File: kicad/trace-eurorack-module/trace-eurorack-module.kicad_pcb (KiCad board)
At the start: 2 copper layers, 7 parts, among them J1 Eurorack_Power, U1 AP63203WU-7

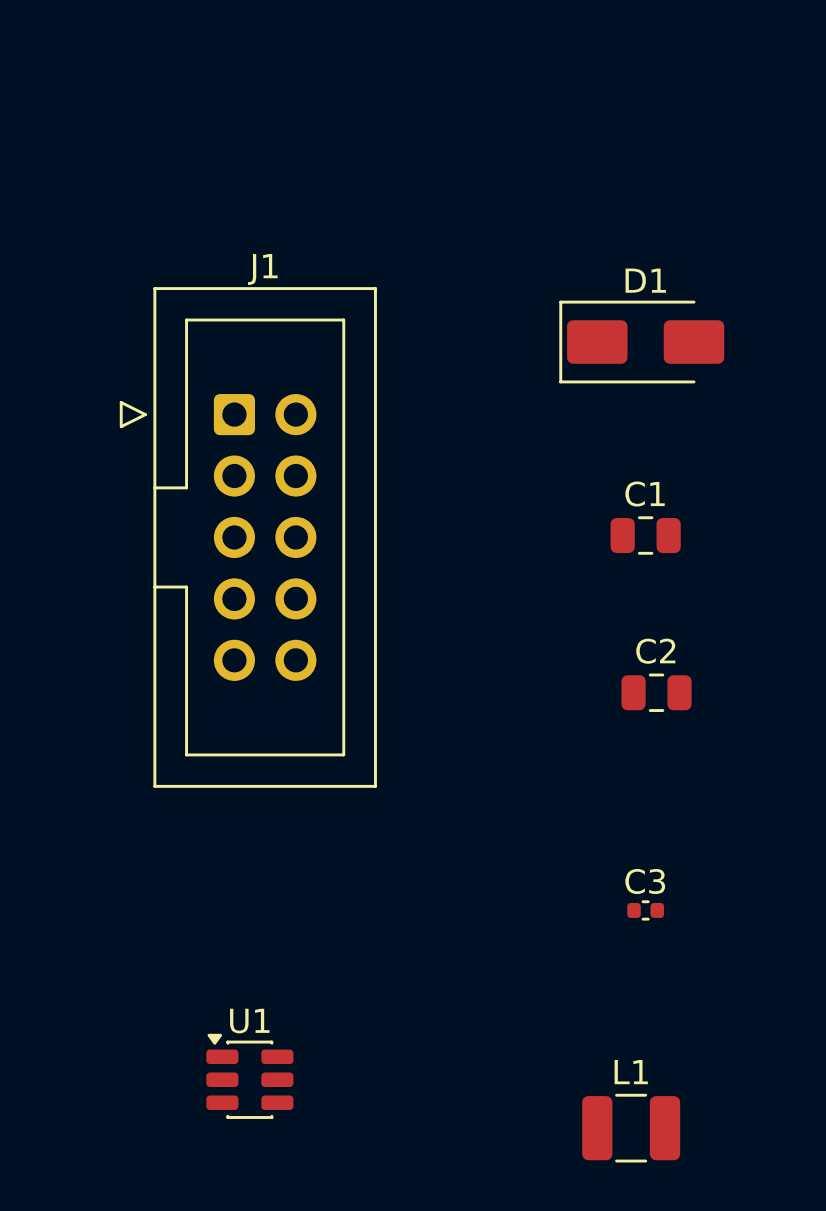
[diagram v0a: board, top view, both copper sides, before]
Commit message: saved
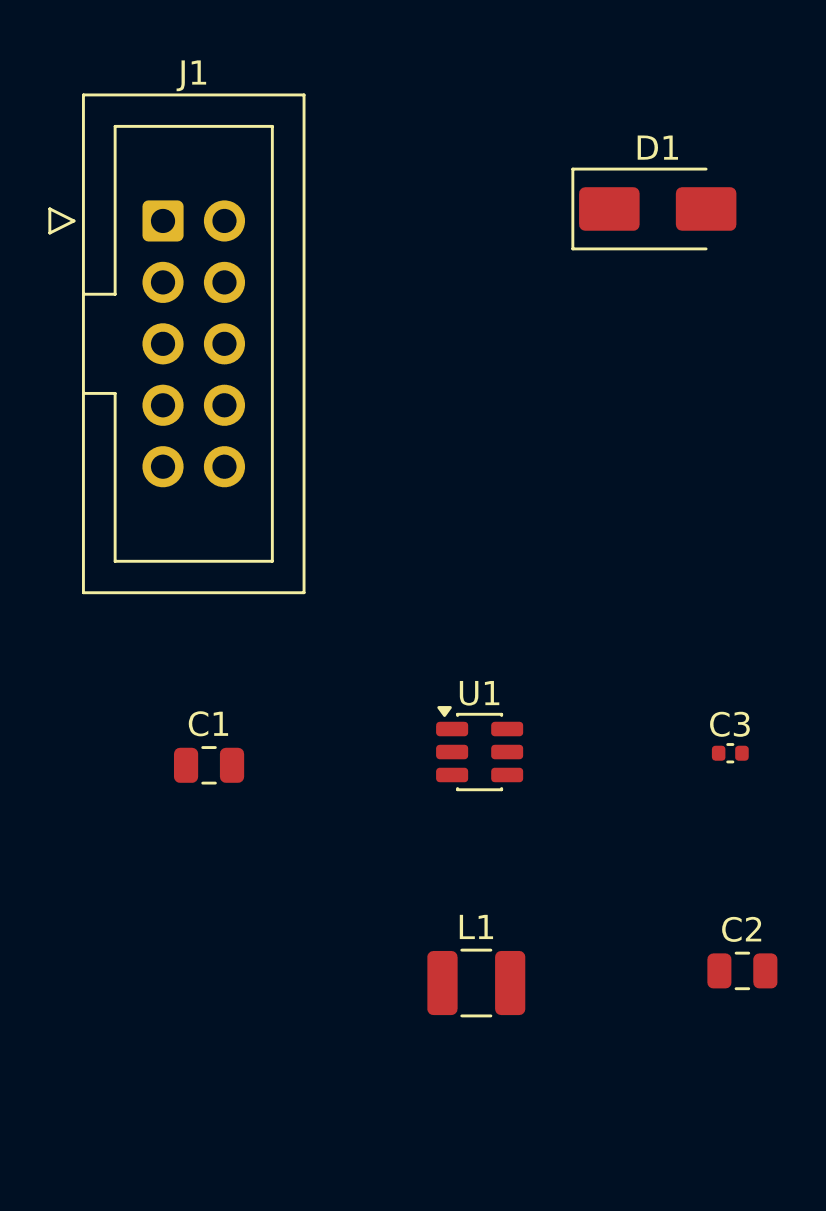
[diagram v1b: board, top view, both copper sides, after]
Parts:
- moved C1 20.4 mm to (26.9, 44.0)
- moved U1 16.5 mm to (38.1, 43.5)
- moved C2 12.0 mm to (49.0, 52.5)
- moved L1 8.77 mm to (38.0, 53.0)
- moved J1 8.53 mm to (25.0, 21.5)
- moved C3 7.38 mm to (48.5, 43.5)
- moved D1 5.52 mm to (45.5, 21.0)
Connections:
- net N$1 renamed -12V_RAW
- net N$2 renamed BST
